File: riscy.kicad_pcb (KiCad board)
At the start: 2 copper layers, 36 parts, among them J1 Conn_01x15_Pin, J2 Conn_01x15_Pin, J3 USB_C_Receptacle_USB2.0_14P, Q1 MMBT2222A, Q2 MMBT2222A, SW1 SW_MEC_5E, SW3 SW_MEC_5E, U2 FT231XS, U3 ESP32-C3-WROOM-02, U4 AMS1117-3.3

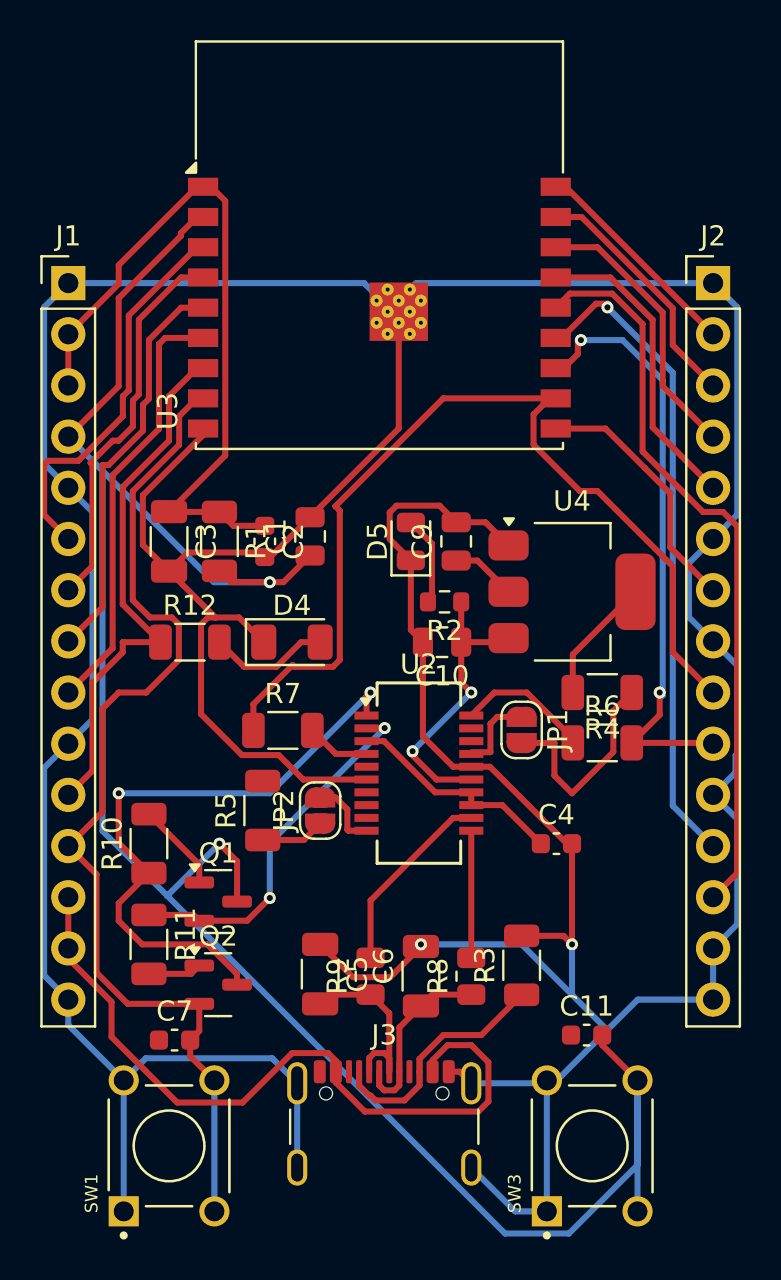
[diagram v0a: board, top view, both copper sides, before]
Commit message: updated
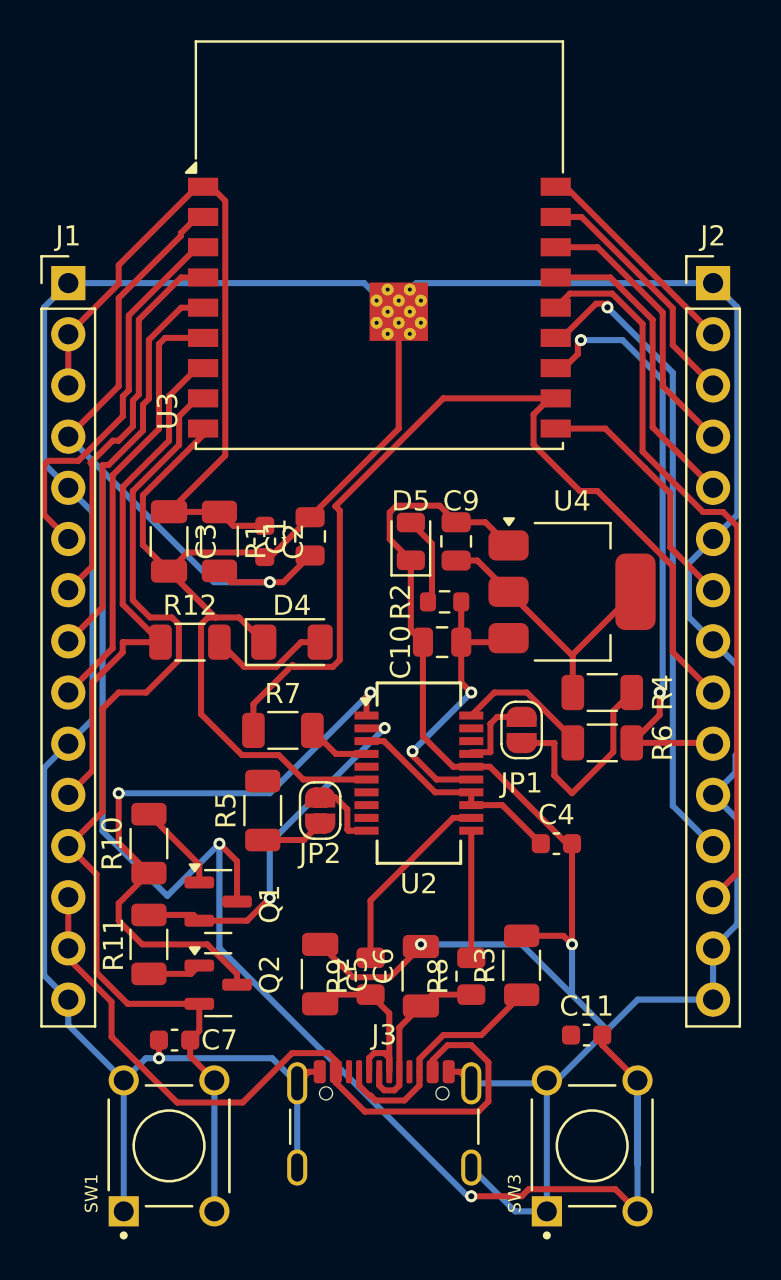
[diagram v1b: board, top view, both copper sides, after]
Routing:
- net +3V3: track 45.3 -> 49.8 mm
- net GND: track 268.0 -> 270.3 mm, vias 2 -> 3
- net /EN: track 106.8 -> 106.7 mm, vias 2 -> 3
